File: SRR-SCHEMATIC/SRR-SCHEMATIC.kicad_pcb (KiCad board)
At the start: 2 copper layers, 113.9 x 75.4 mm, 62 parts, among them J1 Screw_Terminal_01x02, J2 Conn_01x05, SW2 SW_Push, U1 STM32F411CEUx, U2 NCP1117ST50T3G, U3 NCP1117ST33T3G, U4 NHD-C0220BIZ, U5 VL53L1CXV0FY1, U6 VL53L1CXV0FY1, Y1 16MHz

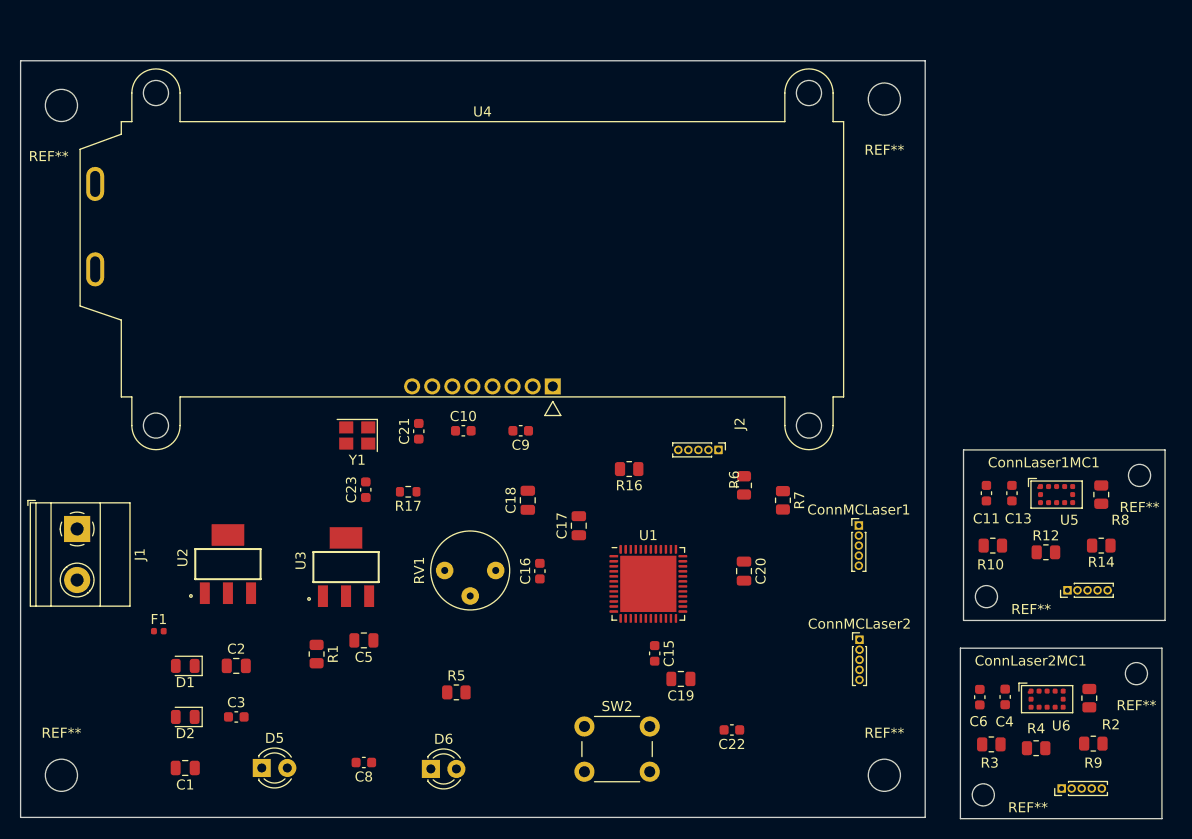
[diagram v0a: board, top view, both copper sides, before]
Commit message: Subindo PCB Corrigida
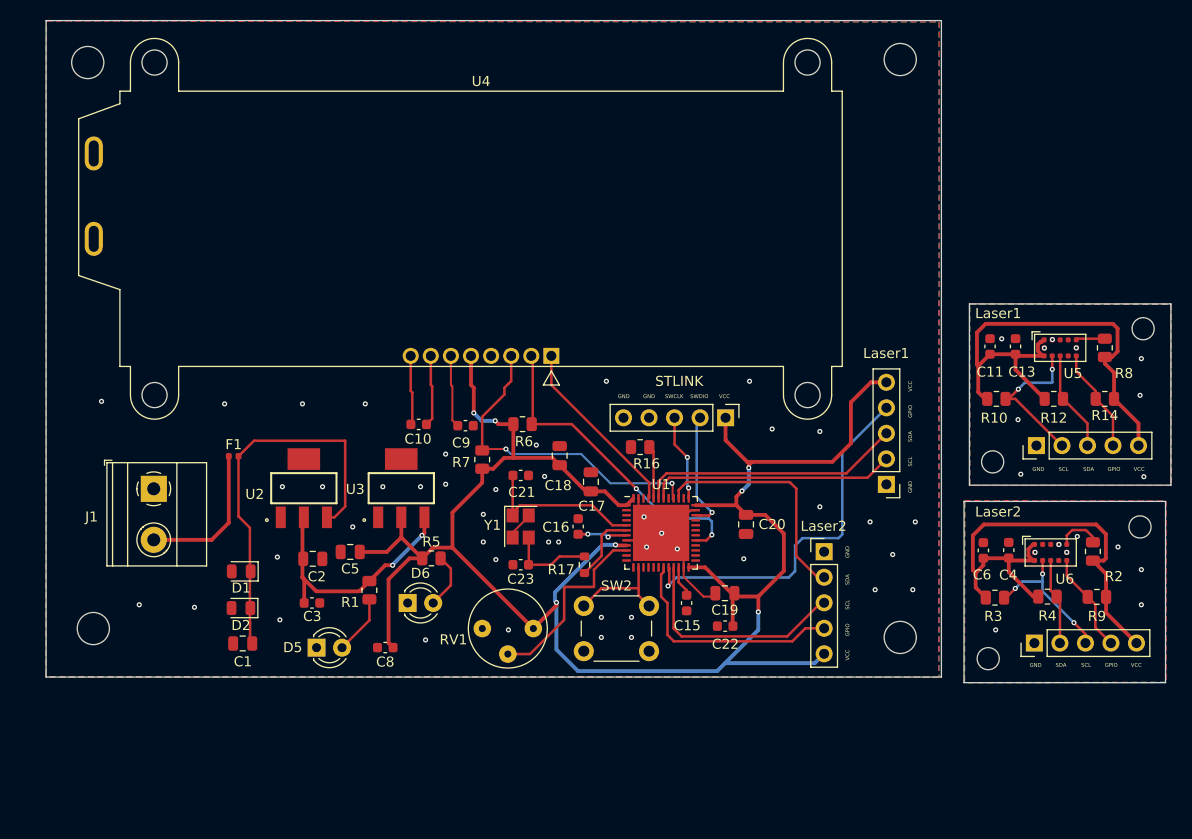
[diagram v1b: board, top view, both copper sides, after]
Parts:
- Laser1: renamed from ConnMCLaser1; footprint Connector_PinHeader_1.00mm:PinHeader_1x05_P1.00mm_Vertical -> Connector_PinHeader_2.54mm:PinHeader_1x05_P2.54mm_Vertical
- Laser1: renamed from ConnLaser1MC1; footprint Connector_PinHeader_1.00mm:PinHeader_1x05_P1.00mm_Vertical -> Connector_PinHeader_2.54mm:PinHeader_1x05_P2.54mm_Vertical
- Laser2: renamed from ConnLaser2MC1; footprint Connector_PinHeader_1.00mm:PinHeader_1x05_P1.00mm_Vertical -> Connector_PinHeader_2.54mm:PinHeader_1x05_P2.54mm_Vertical
- Laser2: renamed from ConnMCLaser2; footprint Connector_PinHeader_1.00mm:PinHeader_1x05_P1.00mm_Vertical -> Connector_PinHeader_2.54mm:PinHeader_1x05_P2.54mm_Vertical
- STLINK: renamed from J2; footprint Connector_PinHeader_1.00mm:PinHeader_1x05_P1.00mm_Vertical -> Connector_PinHeader_2.54mm:PinHeader_1x05_P2.54mm_Vertical
- moved R7 30.2 mm to (145.4, 77.8), turned to 90 degrees
- moved R6 22.9 mm to (149.4, 74.3), turned to 0 degrees
- moved R17 19.0 mm to (155.6, 88.3), turned to 90 degrees
- moved F1 18.9 mm to (120.7, 77.5)
- moved Y1 18.6 mm to (149.2, 84.5), turned to -90 degrees
- moved C23 17.1 mm to (149.2, 88.3), turned to 180 degrees
- moved D6 16.7 mm to (138.0, 92.1)
- moved R12 15.3 mm to (202.3, 71.8)
- moved R4 15.1 mm to (201.7, 91.4)
- moved REF** 14.9 mm to (106.7, 94.6)
- moved Laser1 14.7 mm to (200.6, 76.4)
- moved Laser2 14.7 mm to (200.4, 96.1)
- moved C11 14.6 mm to (195.9, 66.5)
- moved C13 14.6 mm to (198.5, 66.5)
- moved C4 14.6 mm to (197.8, 86.8)
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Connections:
- Laser1 pad 2: I2C1_SDA_LASER1 -> I2C1_SCL_LASER1
- Laser1 pad 3: I2C1_SCL_LASER1 -> I2C1_SDA_LASER1
- R10 pad 2: Net-(ConnLaser1MC1-Pad3) -> Net-(ConnLaser1MC1-Pad2)
- R12 pad 2: Net-(ConnLaser1MC1-Pad2) -> Net-(ConnLaser1MC1-Pad3)
- U1 pad 13: RESET_NHD -> unconnected-(U1-Pad13)
- U1 pad 29: unconnected-(U1-Pad29) -> I2C3_SCL_NHD
- U1 pad 45: I2C3_SCL_NHD -> RESET_NHD
- U5 pad 10: Net-(ConnLaser1MC1-Pad3) -> Net-(ConnLaser1MC1-Pad2)
- U5 pad 9: Net-(ConnLaser1MC1-Pad2) -> Net-(ConnLaser1MC1-Pad3)
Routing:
- net +3V3: track 0.00 -> 189.5 mm, vias 0 -> 7
- net +3.3VADC: track 0.00 -> 50.5 mm
- net +3.3VDAC: track 0.00 -> 49.3 mm
- net Net-(C1-Pad1): track 0.00 -> 39.6 mm
- net GPIO1_LASER1: track 0.00 -> 37.3 mm, vias 0 -> 1
- net I2C3_SDA_NHD: track 0.00 -> 32.6 mm, vias 0 -> 2
- net I2C3_SCL_NHD: track 0.00 -> 32.0 mm, vias 0 -> 2
- net I2C1_SDA_LASER1: track 0.00 -> 26.4 mm
- net GNDREF: track 0.00 -> 25.8 mm, vias 0 -> 44
- net +5V: track 0.00 -> 25.4 mm, vias 0 -> 2
- net I2C1_SCL_LASER1: track 0.00 -> 24.7 mm
- net I2C2_SDA_LASER2: track 0.00 -> 23.5 mm
- net GPIO1_LASER2: track 0.00 -> 23.5 mm
- net I2C2_SCL_LASER2: track 0.00 -> 22.6 mm
- net DISTANCE_REGULATOR: track 0.00 -> 18.9 mm
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- added copper zone on B.Cu, net GND
- added copper zone on F.Cu, net GND
- added copper zone on B.Cu, net GND2
- added copper zone on F.Cu, net GND2
- added copper zone on B.Cu, net GNDREF
- added copper zone on F.Cu, net GNDREF
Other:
- board size 113.9 x 75.4 mm -> 112 x 65.9 mm
- board text added: "GND"
- board text added: "GPIO"
- board text added: "SCL"
- board text added: "SDA"
- board text added: "SWCLK"
- board text added: "SWDIO"
- board text added: "VCC"
